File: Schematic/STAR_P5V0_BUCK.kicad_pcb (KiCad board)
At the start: 2 copper layers, 21 parts, among them J1 1017491, J2 1017491, U1 TPS566238PRQFR

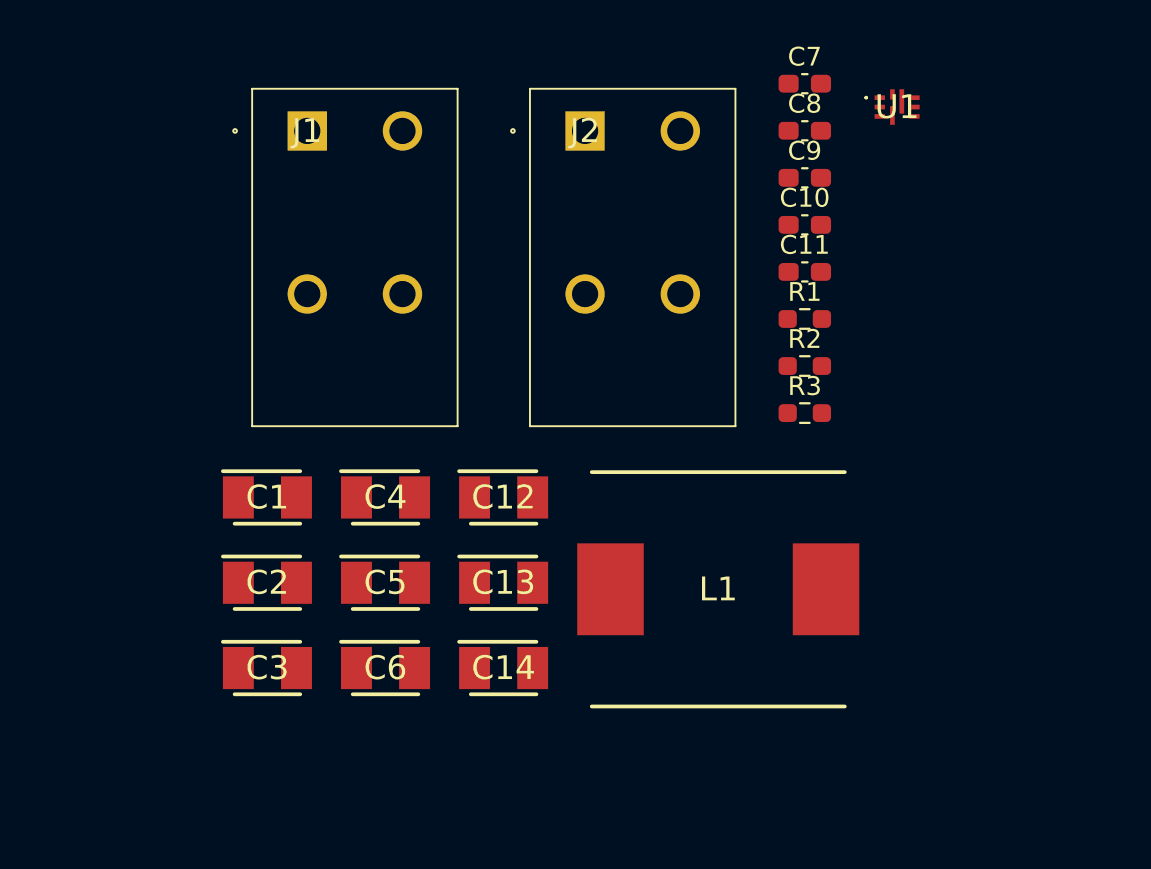
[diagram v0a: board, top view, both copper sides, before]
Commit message: updated schematic
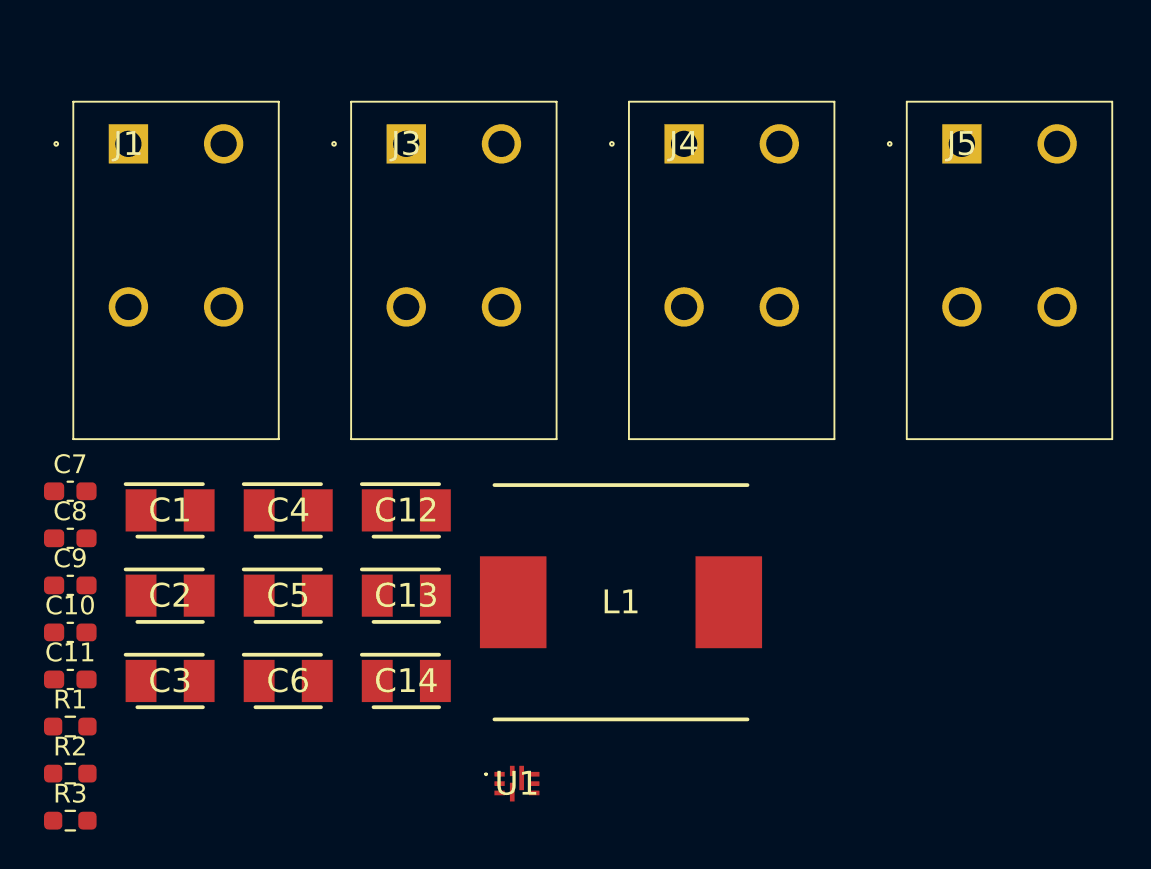
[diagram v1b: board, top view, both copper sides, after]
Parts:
- removed J2: 1017491, 1017491:1017491
- added J3: 1017491, 1017491:1017491, F.Cu at (122.3, 70.9)
- added J4: 1017491, 1017491:1017491, F.Cu at (137.1, 70.9)
- added J5: 1017491, 1017491:1017491, F.Cu at (151.9, 70.9)
- moved C10 44.8 mm to (104.4, 96.9)
- moved C7 44.8 mm to (104.4, 89.4)
- moved R1 44.8 mm to (104.4, 102.0)
- moved C11 44.8 mm to (104.4, 99.4)
- moved C8 44.8 mm to (104.4, 91.9)
- moved C9 44.8 mm to (104.4, 94.4)
- moved R2 44.8 mm to (104.4, 104.5)
- moved R3 44.8 mm to (104.4, 107.0)
- moved U1 41.4 mm to (128.2, 105.0)
- moved J1 9.56 mm to (107.5, 70.9)
- moved C1 5.24 mm to (109.7, 90.4)
- moved C2 5.24 mm to (109.7, 95.0)
- moved C3 5.24 mm to (109.7, 99.5)
- moved C12 5.24 mm to (122.3, 90.4)
- moved C13 5.24 mm to (122.3, 95.0)
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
